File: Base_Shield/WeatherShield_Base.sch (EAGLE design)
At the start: 73 parts, among them Q1 BSS138, Q2 BSS138, U1 DS3231SN, U2 LT3652, U3 TMP100MDBVREP, U4 ADS1015IDGST

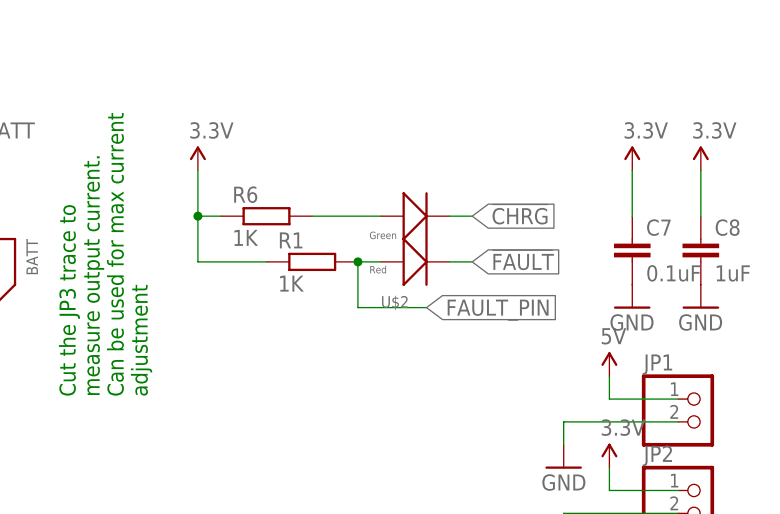
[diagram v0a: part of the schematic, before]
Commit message: WeatherShield_v1
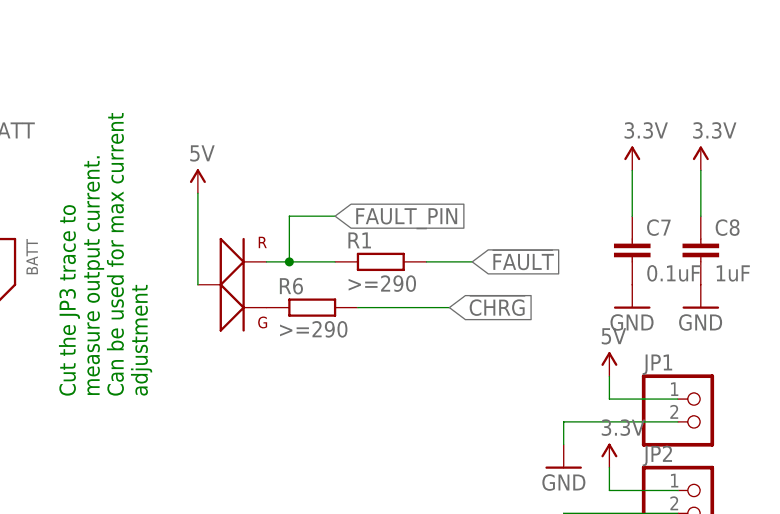
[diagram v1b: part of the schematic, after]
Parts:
- removed U$2: HSMF_C158, FSEWeatherShield:HSMF_C158
- added U$3: VLMV3100, FSEWeatherShield:VLMV3100
- R1, R6: value 1K -> >=290
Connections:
- removed net N$7: R6.2, U$2.1
- new net N$4: R6.1, U$3.3
- net !CHRG: now also R6.2; no longer U$2.2
- net !FAULT: now also R1.2; no longer U$2.4
- net 3.3V: no longer R1.1, R6.1
- net 5V: now also U$3.1
- net FAULT_PIN: now also R1.1, U$3.2; no longer R1.2, U$2.3
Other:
- moved on the sheet: R1, R6
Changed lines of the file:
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@@
 </classes>
 <parts>
-<part name="R6" library="rcl" deviceset="R-EU_" device="R0603" value="1K"/>
-<part name="R1" library="rcl" deviceset="R-EU_" device="R0603" value="1K"/>
+<part name="R6" library="rcl" deviceset="R-EU_" device="R0603" value="&gt;=290"/>
+<part name="R1" library="rcl" deviceset="R-EU_" device="R0603" value="&gt;=290"/>
 <part name="C7" library="rcl" deviceset="C-EU" device="C0603" value="0.1uF"/>
 <part name="GND7" library="SparkFun" deviceset="GND" device=""/>
@@
 <part name="RTCBAT" library="FSEWeatherShield" deviceset="BATTERIE_HALTER_CR1225" device="" value="CR1225"/>
 <part name="U$1" library="FSEWeatherShield" deviceset="POT_TS63Y_10K" device="" value="POT10K"/>
-<part name="U$2" library="FSEWeatherShield" deviceset="HSMF_C158" device=""/>
-<part name="P+12" library="SparkFun" deviceset="3.3V" device=""/>
 <part name="P+3" library="SparkFun" deviceset="3.3V" device=""/>
 <part name="P+10" library="SparkFun" deviceset="3.3V" device=""/>
 <part name="P+13" library="SparkFun" deviceset="3.3V" device=""/>
 <part name="P+1" library="SparkFun" deviceset="3.3V" device=""/>
+<part name="U$3" library="FSEWeatherShield" deviceset="VLMV3100" device=""/>
+<part name="SUPPLY5" library="SparkFun-Aesthetics" deviceset="5V" device=""/>
 </parts>
 <sheets>
@@
 </plain>
 <instances>
-<instance part="R6" gate="G$1" x="210.82" y="167.64"/>
-<instance part="R1" gate="G$1" x="215.9" y="162.56"/>
+<instance part="R6" gate="G$1" x="215.9" y="157.48"/>
+<instance part="R1" gate="G$1" x="223.52" y="162.56"/>
 <instance part="C7" gate="G$1" x="251.46" y="165.1"/>
 <instance part="GND7" gate="1" x="251.46" y="157.48"/>
@@
 <instance part="RTCBAT" gate="G$1" x="121.92" y="88.9"/>
 <instance part="U$1" gate="G$1" x="25.4" y="152.4"/>
-<instance part="U$2" gate="G$1" x="226.06" y="165.1"/>
-<instance part="P+12" gate="G$1" x="203.2" y="172.72"/>
 <instance part="P+3" gate="G$1" x="251.46" y="172.72"/>
 <instance part="P+10" gate="G$1" x="259.08" y="172.72"/>
 <instance part="P+13" gate="G$1" x="175.26" y="114.3"/>
 <instance part="P+1" gate="G$1" x="129.54" y="99.06"/>
+<instance part="U$3" gate="G$1" x="205.74" y="160.02"/>
+<instance part="SUPPLY5" gate="G$1" x="203.2" y="170.18"/>
 </instances>
 <busses>
@@
 </segment>
 </net>
-<net name="N$7" class="0">
-<segment>
-<wire x1="215.9" y1="167.64" x2="223.52" y2="167.64" width="0.1524" layer="91"/>
-<pinref part="R6" gate="G$1" pin="2"/>
-<pinref part="U$2" gate="G$1" pin="1"/>
-</segment>
-</net>
 <net name="FAULT_PIN" class="0">
 <segment>
-<wire x1="223.52" y1="162.56" x2="220.98" y2="162.56" width="0.1524" layer="91"/>
-<pinref part="R1" gate="G$1" pin="2"/>
-<wire x1="220.98" y1="162.56" x2="220.98" y2="157.48" width="0.1524" layer="91"/>
-<junction x="220.98" y="162.56"/>
-<wire x1="220.98" y1="157.48" x2="228.6" y2="157.48" width="0.1524" layer="91"/>
-<label x="228.6" y="157.48" size="1.778" layer="95" xref="yes"/>
-<pinref part="U$2" gate="G$1" pin="3"/>
+<label x="218.44" y="167.64" size="1.778" layer="95" xref="yes"/>
+<pinref part="R1" gate="G$1" pin="1"/>
+<pinref part="U$3" gate="G$1" pin="2"/>
+<wire x1="218.44" y1="162.56" x2="213.36" y2="162.56" width="0.1524" layer="91"/>
+<wire x1="213.36" y1="162.56" x2="210.82" y2="162.56" width="0.1524" layer="91"/>
+<wire x1="218.44" y1="167.64" x2="213.36" y2="167.64" width="0.1524" layer="91"/>
+<wire x1="213.36" y1="167.64" x2="213.36" y2="162.56" width="0.1524" layer="91"/>
+<junction x="213.36" y="162.56"/>
 </segment>
 <segment>
@@
 <wire x1="12.7" y1="91.44" x2="20.32" y2="91.44" width="0.1524" layer="91"/>
 <wire x1="20.32" y1="91.44" x2="20.32" y2="104.14" width="0.1524" layer="91"/>
-</segment>
-<segment>
-<wire x1="203.2" y1="172.72" x2="203.2" y2="167.64" width="0.1524" layer="91"/>
-<pinref part="R6" gate="G$1" pin="1"/>
-<wire x1="203.2" y1="167.64" x2="203.2" y2="162.56" width="0.1524" layer="91"/>
-<wire x1="205.74" y1="167.64" x2="203.2" y2="167.64" width="0.1524" layer="91"/>
-<pinref part="R1" gate="G$1" pin="1"/>
-<wire x1="210.82" y1="162.56" x2="203.2" y2="162.56" width="0.1524" layer="91"/>
-<junction x="203.2" y="167.64"/>
-<pinref part="P+12" gate="G$1" pin="3.3V"/>
 </segment>
 <segment>
@@
 <junction x="58.42" y="104.14"/>
 </segment>
+<segment>
+<pinref part="U$3" gate="G$1" pin="1"/>
+<wire x1="203.2" y1="170.18" x2="203.2" y2="160.02" width="0.1524" layer="91"/>
+<pinref part="SUPPLY5" gate="G$1" pin="5V"/>
+</segment>
 </net>
 <net name="RAIN" class="0">
@@
 </segment>
 <segment>
-<label x="233.68" y="167.64" size="1.778" layer="95" xref="yes"/>
-<wire x1="233.68" y1="167.64" x2="231.14" y2="167.64" width="0.1524" layer="91"/>
-<pinref part="U$2" gate="G$1" pin="2"/>
+<label x="231.14" y="157.48" size="1.778" layer="95" xref="yes"/>
+<wire x1="231.14" y1="157.48" x2="220.98" y2="157.48" width="0.1524" layer="91"/>
+<pinref part="R6" gate="G$1" pin="2"/>
 </segment>
 </net>
@@
 <segment>
 <label x="233.68" y="162.56" size="1.778" layer="95" xref="yes"/>
-<wire x1="233.68" y1="162.56" x2="231.14" y2="162.56" width="0.1524" layer="91"/>
-<pinref part="U$2" gate="G$1" pin="4"/>
+<pinref part="R1" gate="G$1" pin="2"/>
+<wire x1="228.6" y1="162.56" x2="233.68" y2="162.56" width="0.1524" layer="91"/>
 </segment>
 </net>
@@
 </segment>
 </net>
+<net name="N$4" class="0">
+<segment>
+<pinref part="U$3" gate="G$1" pin="3"/>
+<pinref part="R6" gate="G$1" pin="1"/>
+</segment>
+</net>

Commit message: WeatherShield_v1
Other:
- note added: "Raspberry Pi"
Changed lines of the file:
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@@
 <sheet>
 <plain>
-<text x="7.62" y="121.92" size="1.27" layer="98">Wind Speed &amp; Direction</text>
-<text x="147.32" y="134.62" size="1.27" layer="98">Rain sensor</text>
-<text x="142.24" y="101.6" size="1.27" layer="98">RTC Clock</text>
+<text x="7.62" y="121.92" size="1.778" layer="98">Wind Speed &amp; Direction</text>
+<text x="144.78" y="134.62" size="1.778" layer="98">Rain sensor</text>
+<text x="142.24" y="101.6" size="1.778" layer="98">RTC Clock</text>
 <text x="197.612" y="147.574" size="1.778" layer="91" rot="R90">Cut the JP3 trace to
 measure output current.
@@
 <text x="259.08" y="81.28" size="1.778" layer="95" rot="R90">Add. UART</text>
 <text x="172.72" y="71.12" size="1.778" layer="95">Add. SPI</text>
-<text x="154.178" y="8.382" size="2.54" layer="98" rot="R90">Level shifter</text>
-<text x="132.334" y="133.096" size="1.27" layer="98" rot="R180">Air Board Interface</text>
-<text x="68.326" y="174.244" size="1.27" layer="98">Solar cell</text>
+<text x="154.178" y="8.382" size="1.778" layer="98" rot="R90">Level shifter</text>
+<text x="137.414" y="133.096" size="1.778" layer="98" rot="R180">Air Board Interface</text>
+<text x="68.326" y="174.244" size="1.778" layer="98">Solar cell</text>
 <text x="20.32" y="66.04" size="1.27" layer="98">Temperatur sensor</text>
 <text x="116.84" y="55.88" size="1.778" layer="97">7-Bit I2C Address is 0x68</text>
 <text x="20.32" y="63.5" size="1.778" layer="97">7-Bit I2C Address is 0x48</text>
-<text x="68.58" y="106.68" size="1.27" layer="98">ADC 2 I2C</text>
+<text x="68.58" y="106.68" size="1.778" layer="98">ADC 2 I2C</text>
 <wire x1="0" y1="114.3" x2="114.3" y2="114.3" width="0.1524" layer="98" style="longdash"/>
 <wire x1="114.3" y1="114.3" x2="114.3" y2="139.7" width="0.1524" layer="98" style="longdash"/>
@@
 <wire x1="116.84" y1="53.34" x2="170.18" y2="53.34" width="0.1524" layer="98" style="longdash"/>
 <wire x1="116.84" y1="48.26" x2="116.84" y2="0" width="0.1524" layer="98" style="longdash"/>
-<text x="71.12" y="43.18" size="1.27" layer="98">+5V Generation (Raspberry Power)</text>
+<text x="71.12" y="43.18" size="1.778" layer="98">+5V Generation (Raspberry Power)</text>
 <text x="109.22" y="124.46" size="1.778" layer="91" rot="R90">Ubat_float = 13.5V</text>
-<text x="2.54" y="111.76" size="1.27" layer="98">Wind &amp; Wind direction Sensor</text>
+<text x="2.54" y="111.76" size="1.778" layer="98">Wind &amp; Wind direction Sensor</text>
+<text x="190.5" y="124.46" size="1.778" layer="98">Raspberry Pi</text>
 </plain>
 <instances>
